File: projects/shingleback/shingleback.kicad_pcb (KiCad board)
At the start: 2 copper layers, 119.5 x 76 mm, 61 parts

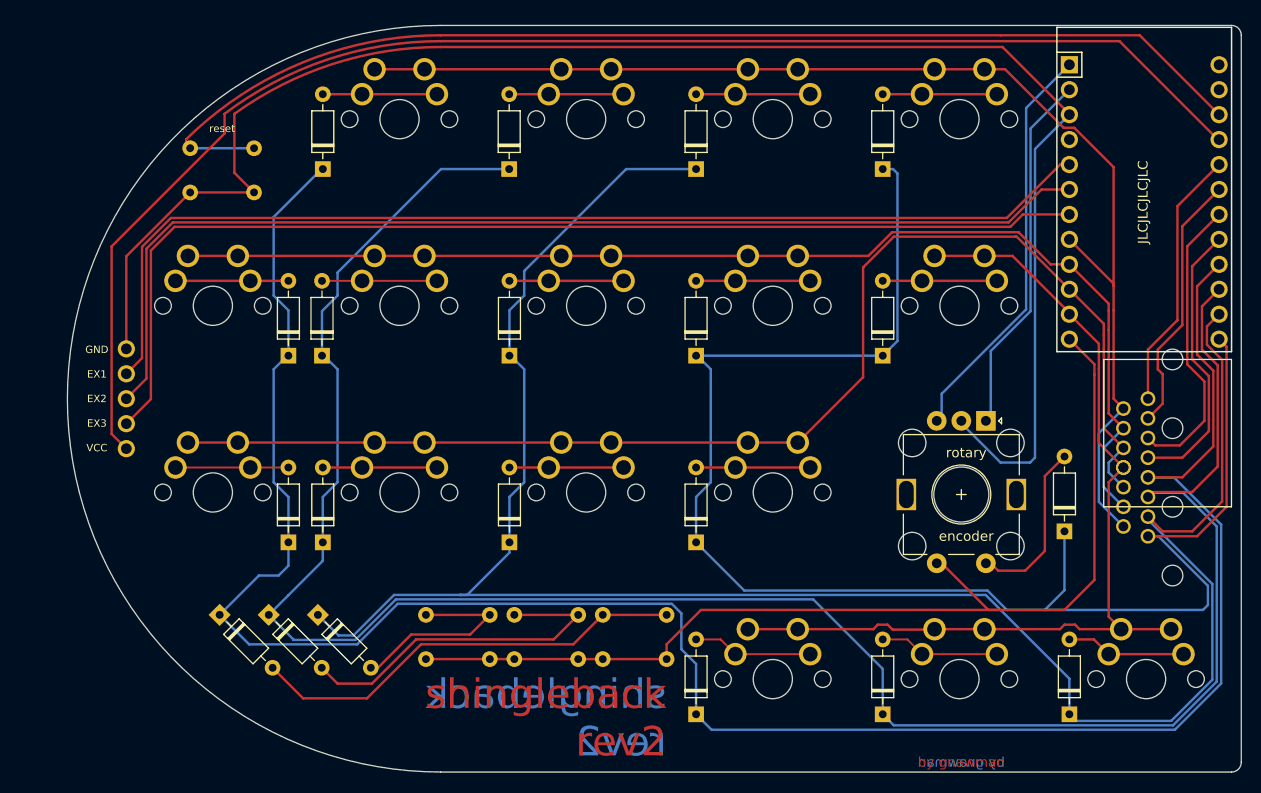
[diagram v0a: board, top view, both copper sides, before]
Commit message: setup for shingleback rev3
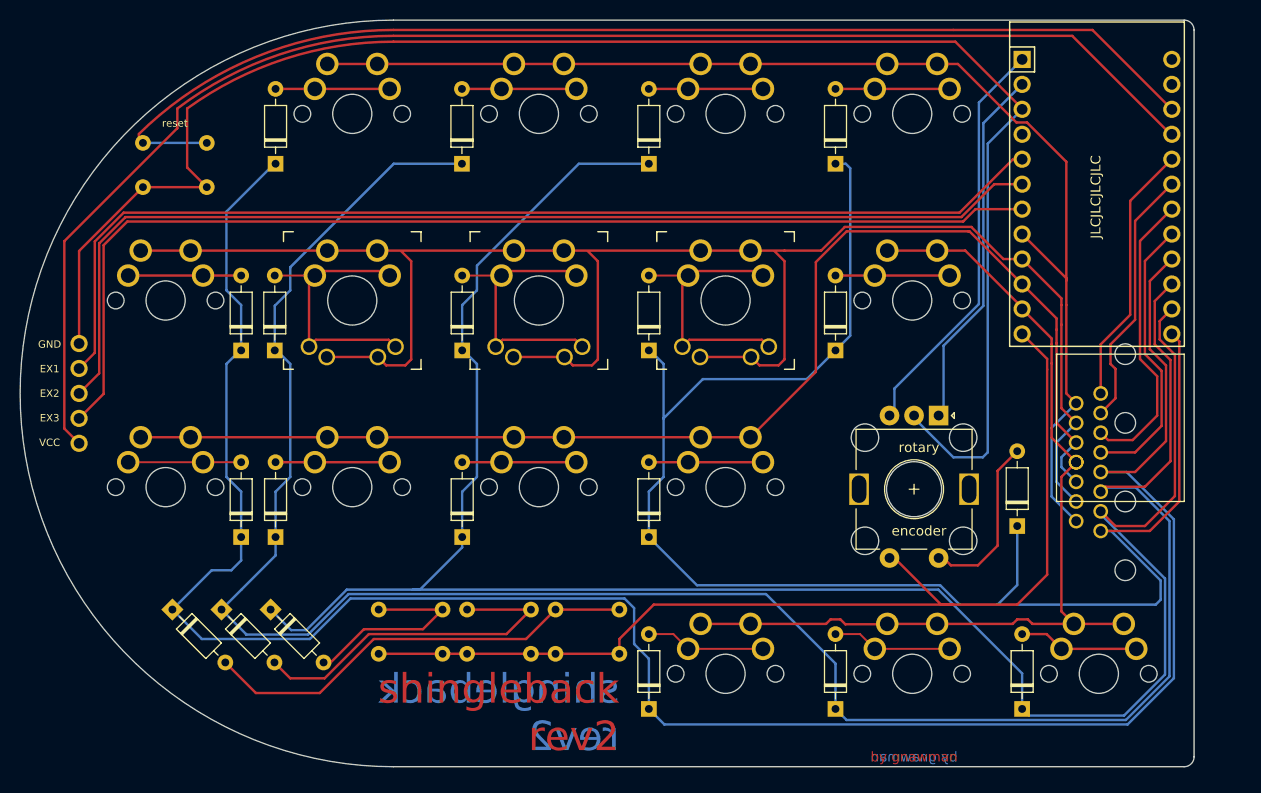
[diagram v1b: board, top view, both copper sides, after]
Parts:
- removed the S14 at (95.8, 69.5)
- removed the S14 at (76.8, 69.5)
- removed the S14 at (57.8, 69.5)
- added s: s, gnawman:Cherry-MX-Gateron-Lo-Flip, F.Cu at (53.0, 69.0)
- added s: s, gnawman:Cherry-MX-Gateron-Lo-Flip, F.Cu at (72.0, 69.0)
- added s: s, gnawman:Cherry-MX-Gateron-Lo-Flip, F.Cu at (91.0, 69.0)
- moved ? 4.84 mm to (71.2, 100.5)
- moved ? 4.84 mm to (71.2, 105.0)
- moved ? 4.84 mm to (55.7, 105.0)
- moved ? 4.84 mm to (64.7, 105.0)
- moved ? 4.84 mm to (62.2, 100.5)
- moved ? 4.84 mm to (55.7, 100.5)
- moved ? 4.84 mm to (73.7, 105.0)
- moved ? 4.84 mm to (64.7, 100.5)
- moved ? 4.84 mm to (80.2, 105.0)
- moved ? 4.84 mm to (73.7, 100.5)
- moved ? 4.84 mm to (62.2, 105.0)
- moved ? 4.84 mm to (80.2, 100.5)
- moved R 4.84 mm to (41.7, 93.1)
- moved R 4.84 mm to (41.7, 74.1)
- moved R 4.84 mm to (102.2, 110.6)
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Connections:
- REF pad : col7 -> col4
- REF pad : col1 -> col3
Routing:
- net row1: track 120.7 -> 182.5 mm
- net (no net): track 306.1 -> 351.8 mm
- net col3: track 160.9 -> 162.3 mm

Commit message: split off skink into separate keb
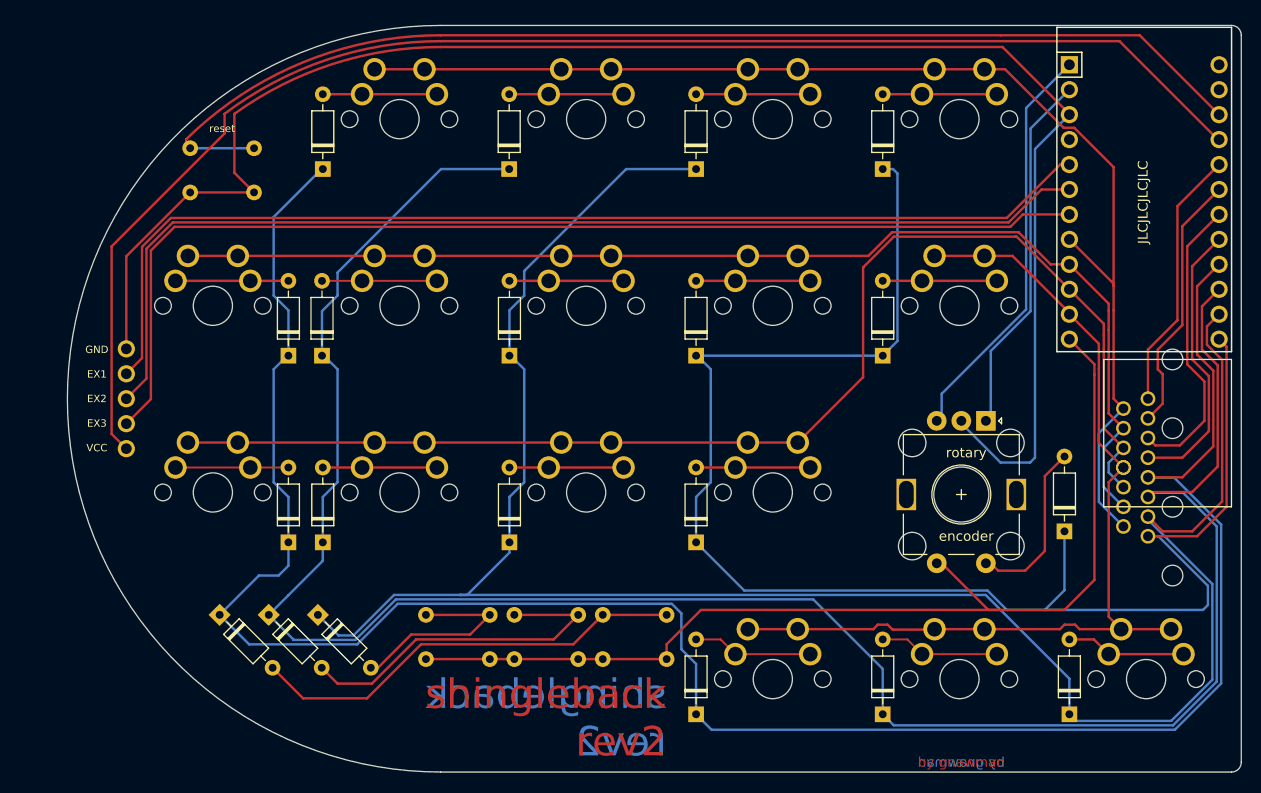
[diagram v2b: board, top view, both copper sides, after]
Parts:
- removed s (x3): s, gnawman:Cherry-MX-Gateron-Lo-Flip
- added S14: , MX, F.Cu at (95.8, 69.5)
- added S14: , MX, F.Cu at (76.8, 69.5)
- added S14: , MX, F.Cu at (57.8, 69.5)
- moved ? 4.84 mm to (76.0, 101.0)
- moved ? 4.84 mm to (76.0, 105.5)
- moved ? 4.84 mm to (60.5, 105.5)
- moved ? 4.84 mm to (69.5, 105.5)
- moved ? 4.84 mm to (67.0, 101.0)
- moved ? 4.84 mm to (60.5, 101.0)
- moved ? 4.84 mm to (78.5, 105.5)
- moved ? 4.84 mm to (69.5, 101.0)
- moved ? 4.84 mm to (85.0, 105.5)
- moved ? 4.84 mm to (78.5, 101.0)
- moved ? 4.84 mm to (67.0, 105.5)
- moved ? 4.84 mm to (85.0, 101.0)
- moved R 4.84 mm to (46.5, 93.6)
- moved R 4.84 mm to (46.5, 74.6)
- moved R 4.84 mm to (107.0, 111.1)
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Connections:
- REF pad : col4 -> col7
- REF pad : col3 -> col1
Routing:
- net row1: track 182.5 -> 120.7 mm
- net (no net): track 351.8 -> 306.1 mm
- net col3: track 162.3 -> 160.9 mm
